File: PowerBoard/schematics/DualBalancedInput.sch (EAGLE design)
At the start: 21 parts, among them IC1 THAT1200, IC2 THAT1646

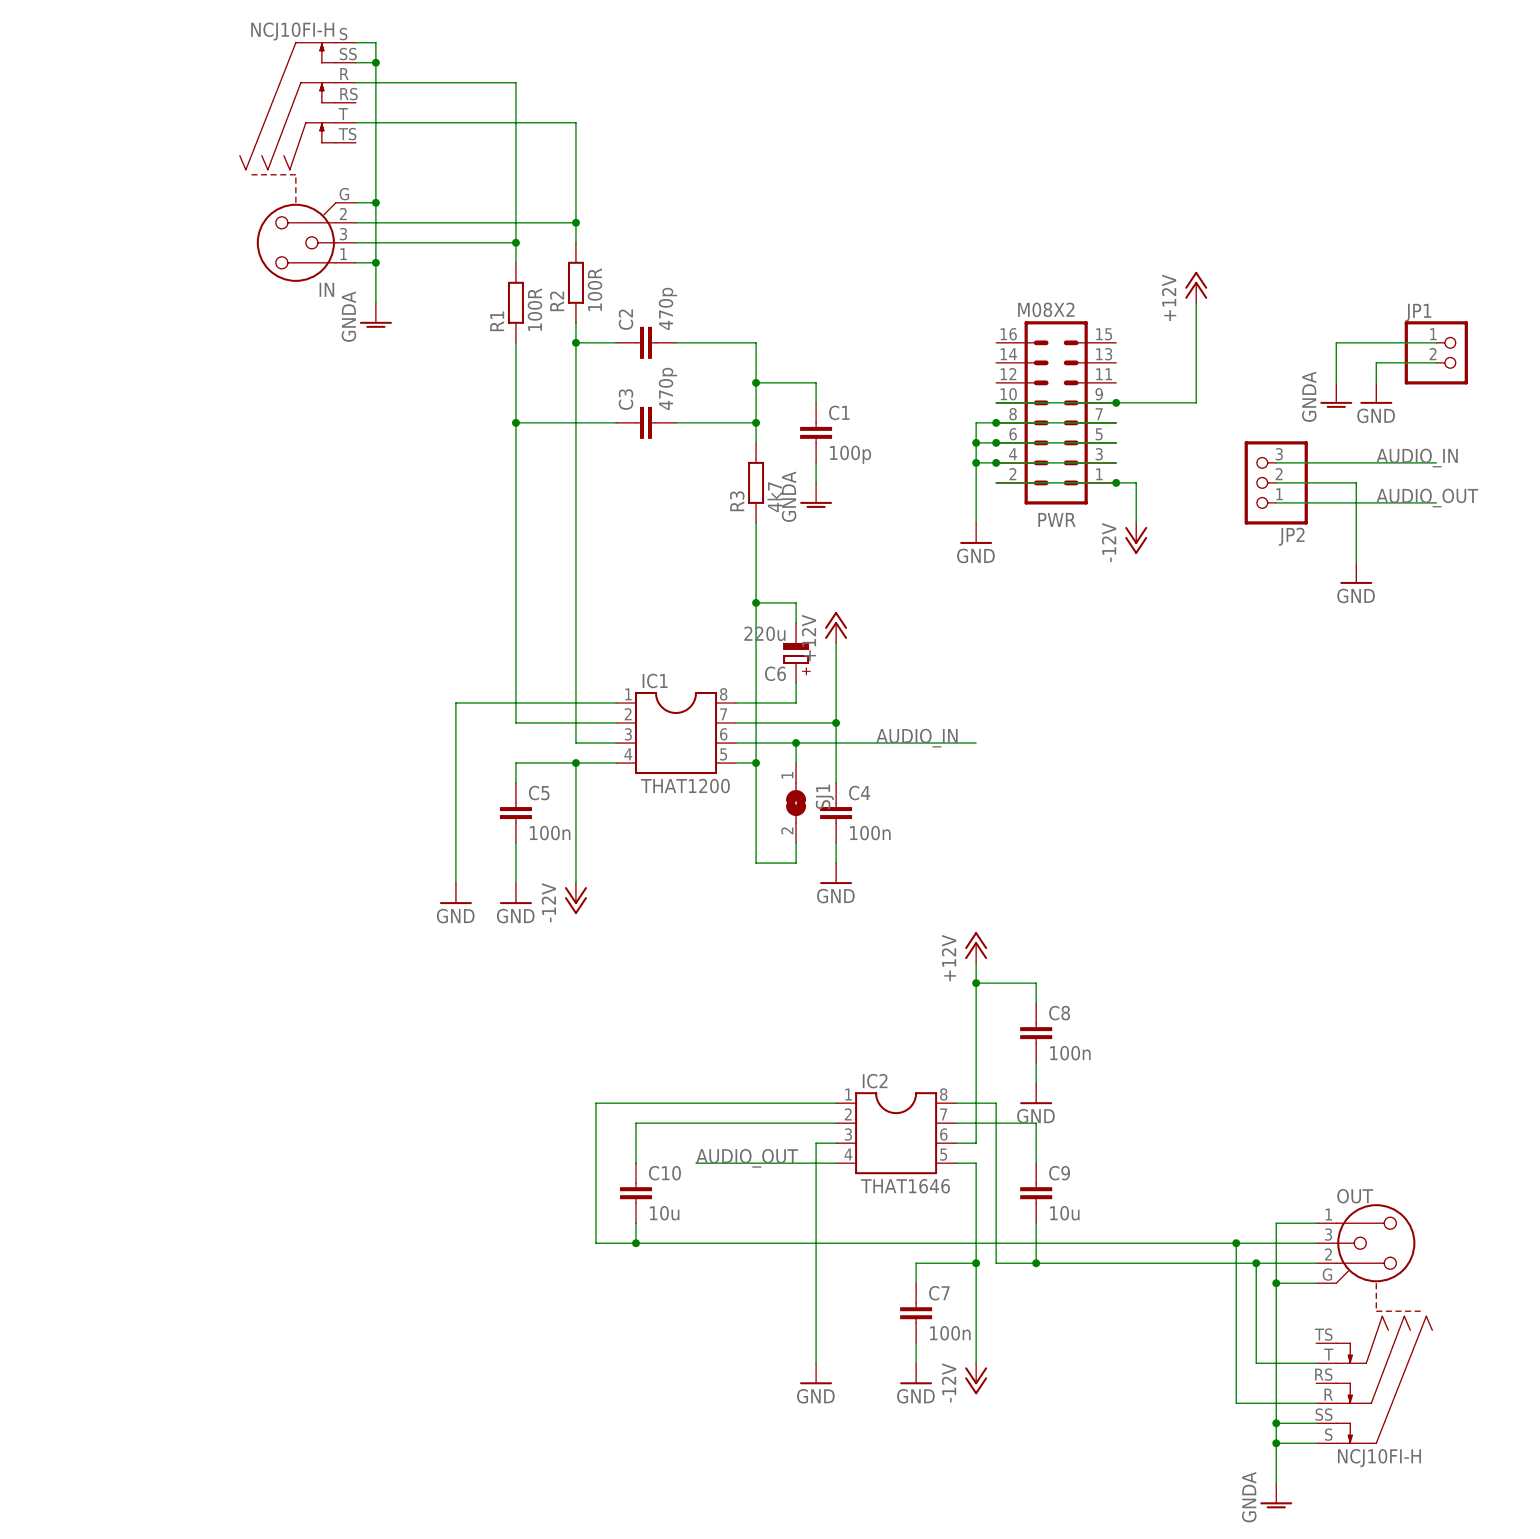
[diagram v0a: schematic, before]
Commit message: latest rev
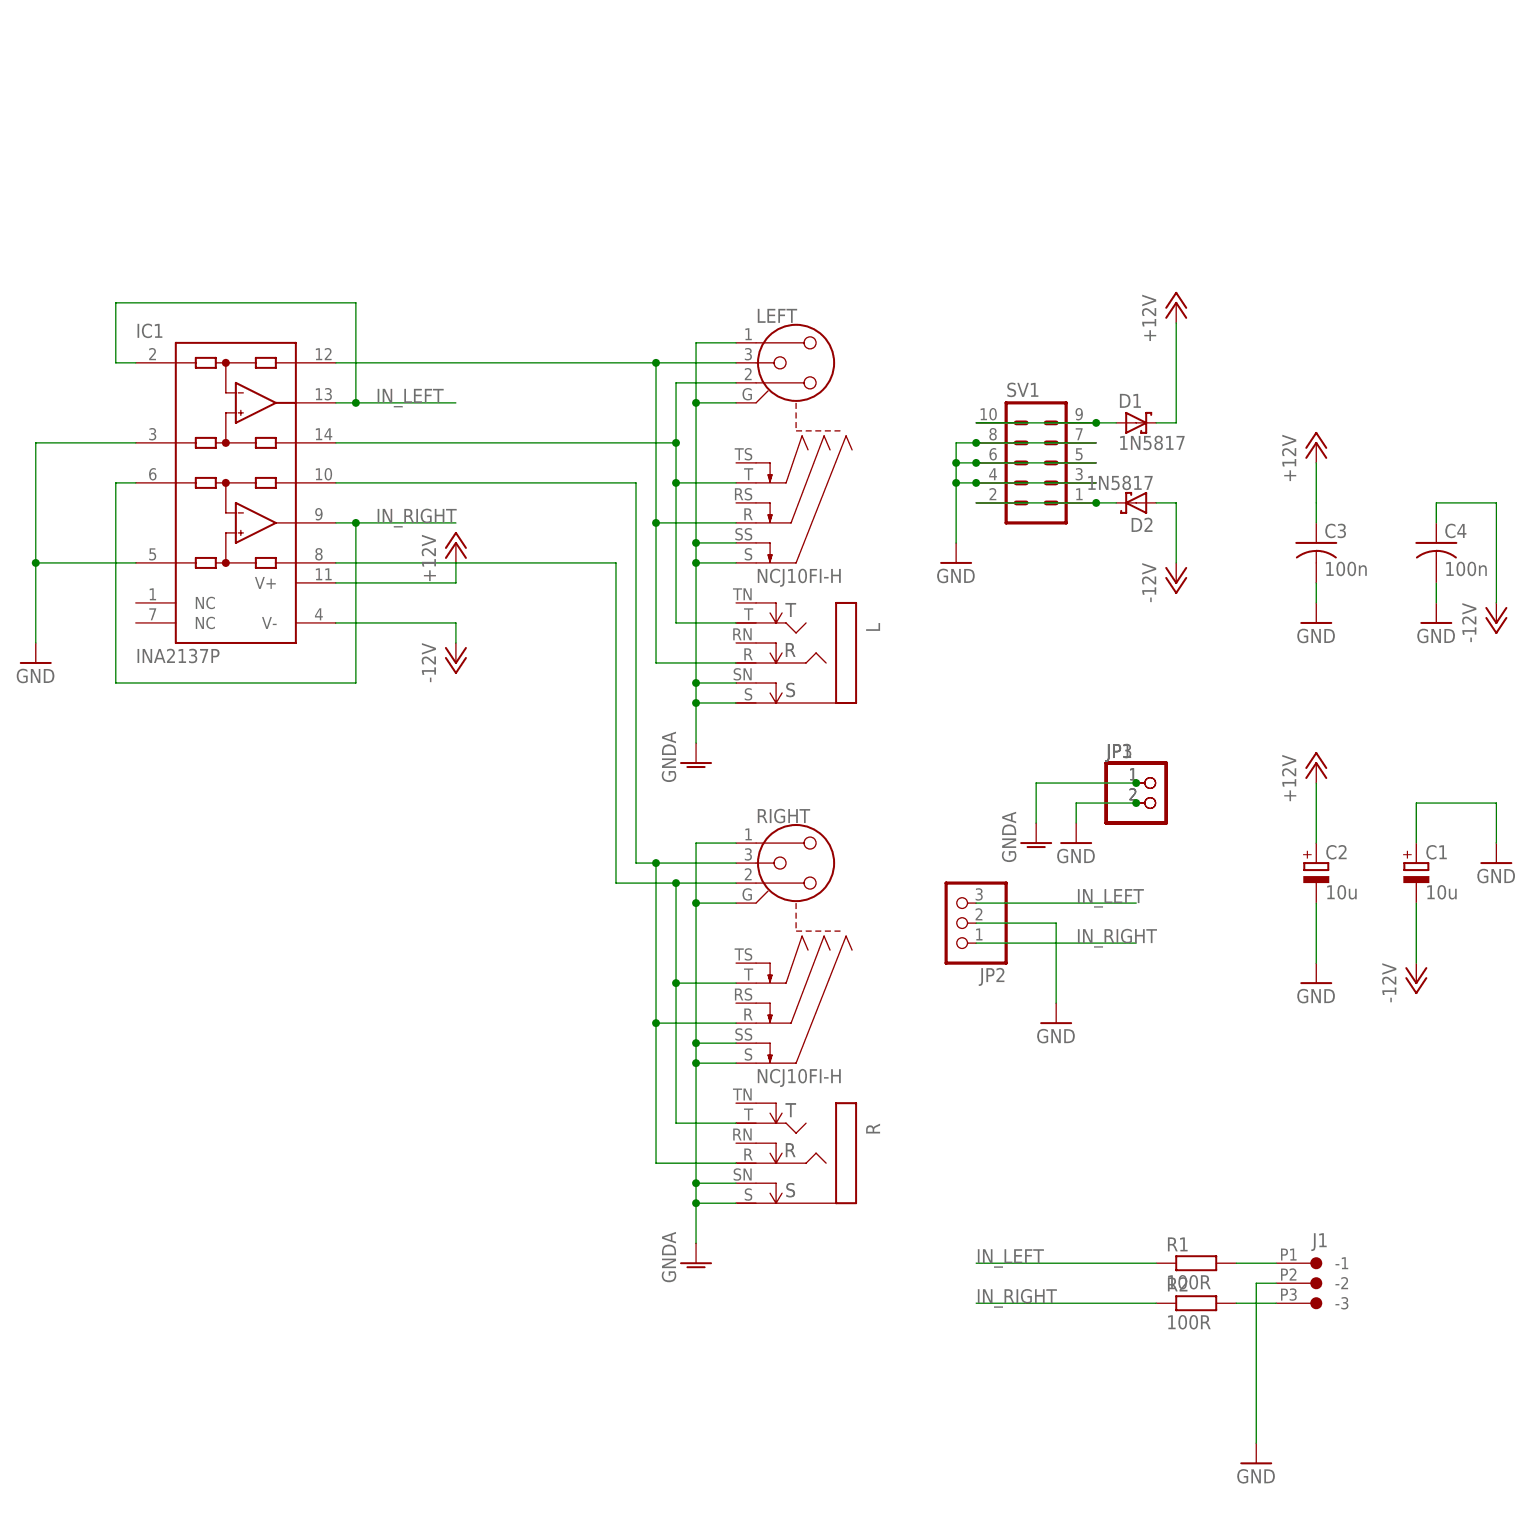
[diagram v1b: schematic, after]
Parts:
- removed C10, C9: 10u, rcl:C-EU050-025X075
- removed C5, C7, C8: 100n, rcl:C-EU050-025X075
- removed C6: 220u, rcl:CPOL-EUE5-8.5
- removed IC2: THAT1646, ic-package:DIL8
- removed IN, OUT: NCJ10FI-H, con-neutrik_ag:NCJ10FI-H
- removed PWR: M08X2, SparkFun:M08X2
- removed R3: 4k7, rcl:R-EU_0207/7
- removed SJ1: (no value), jumper:SJW
- added D1, D2: 1N5817, diode:1N5819-B
- added J1: CON-JST_PH_3W, Rebel:CON-JST_PH_3W
- added JP3: (no value), pinhead:PINHD-1X2
- added L, R: NEUTRIK_NMJ6HCD2, neutrik_jacks:NEUTRIK_NMJ6HCD2
- added LEFT, RIGHT: NCJ10FI-H, con-neutrik_ag:NCJ10FI-H
- added SV1: (no value), con-lstb:MA05-2
- C1: value 100p -> 10u; device rcl:C-EU050-025X075 -> rcl:CPOL-EUE5-6
- C2: value 470p -> 10u; device rcl:C-EU050-025X075 -> rcl:CPOL-EUE5-6
- C3: value 470p -> 100n; device rcl:C-EU050-025X075 -> rcl:C-US050-024X044
- C4: device rcl:C-EU050-025X075 -> rcl:C-US050-024X044
- IC1: value THAT1200 -> INA2137P; device ic-package:DIL8 -> burr-brown:INA2137P
- R1, R2: device rcl:R-EU_0207/7 -> Rebel:R-EU_0204/7
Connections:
- removed net AUDIO_IN: IC1.6, JP2.3, SJ1.1
- removed net AUDIO_OUT: IC2.4, JP2.1
- removed net N$10: C10.1, IC2.2
- removed net N$13: C6.+, IC1.8
- removed net N$3: IN.3, IN.R, R1.2
- removed net N$4: C2.1, IC1.3, R2.1
- removed net N$8: C9.1, IC2.7
- new net IN_LEFT: IC1.-INA, IC1.OUTA, JP2.3, R1.1
- new net IN_RIGHT: IC1.-INB, IC1.OUTB, JP2.1, R2.1
- new net N$2: IC1.SENSEA, L.R, LEFT.3, LEFT.R
- new net N$9: J1.-1, R1.2
- net +12V: now also C2.+, C3.1, D1.C, IC1.V+; no longer C4.1, C8.1, IC1.7, IC2.6, PWR.10, PWR.9
- net -12V: now also C1.-, C4.1, D2.A, IC1.V-; no longer C5.1, C7.1, IC1.4, IC2.5, PWR.1, PWR.2
- net GND: now also C1.+, C2.-, C3.2, IC1.+INA, IC1.+INB, J1.-2, JP3.2, SV1.3, SV1.4, SV1.5, SV1.6, SV1.7, SV1.8; no longer C5.2, C7.2, C8.2, IC1.1, IC2.3, PWR.3, PWR.4, PWR.5, PWR.6, PWR.7, PWR.8
- net GNDA: now also JP3.1, L.S, L.SN, LEFT.1, LEFT.G, LEFT.S, LEFT.SS, R.S, R.SN, RIGHT.1, RIGHT.G, RIGHT.S, RIGHT.SS; no longer C1.2, IN.1, IN.G, IN.S, IN.SS, OUT.1, OUT.G, OUT.S, OUT.SS
- net N$1: now also IC1.REFA, L.T, LEFT.2, LEFT.T; no longer C3.1, IC1.2, R1.1
- net N$18: now also IC1.REFB, R.T, RIGHT.2, RIGHT.T; no longer C9.2, IC2.8, OUT.2, OUT.T
- net N$19: now also IC1.SENSEB, R.R, RIGHT.3, RIGHT.R; no longer C10.2, IC2.1, OUT.3, OUT.R
- net N$5: now also D2.C, SV1.1, SV1.2; no longer IN.2, IN.T, R2.2
- net N$6: now also D1.A, SV1.10, SV1.9; no longer C6.-, IC1.5, R3.1, SJ1.2
- net N$7: now also J1.-3, R2.2; no longer C1.1, C2.2, C3.2, R3.2
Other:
- moved on the sheet: C3, C4, JP1, JP2, R1, R2
